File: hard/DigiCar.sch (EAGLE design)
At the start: 41 parts, among them CN1 EH-2, CN11 ZX62-B-5PA(11), CN2 EH-2, CN3 EH-2, Q1 2SC2712, Q2 2SC2712, SW1 SS-12SDP2, SW2 SKRPACE010, U1 TC1262-3.3VDB, U2 DRV8835, U3 ESP-WROOM-32, U4 FT231XS

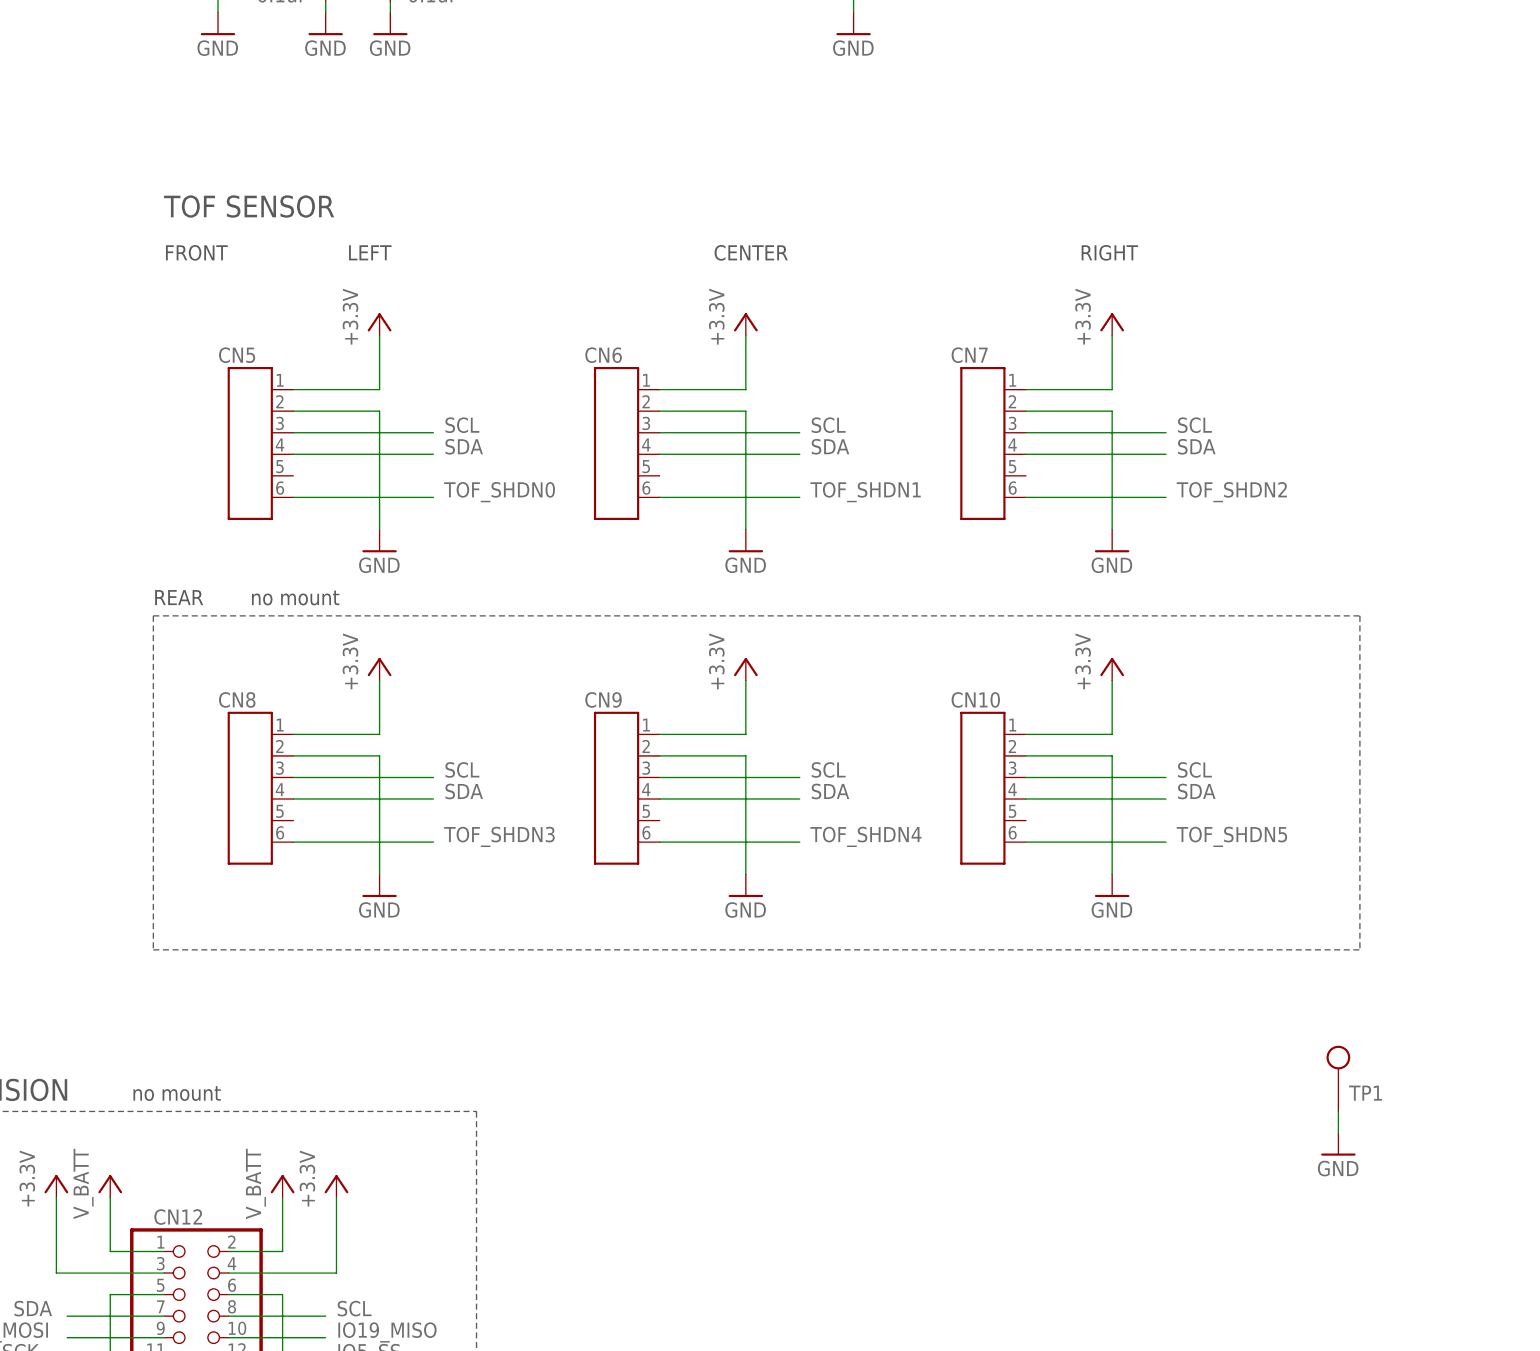
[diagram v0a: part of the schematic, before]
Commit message: 回路を修正
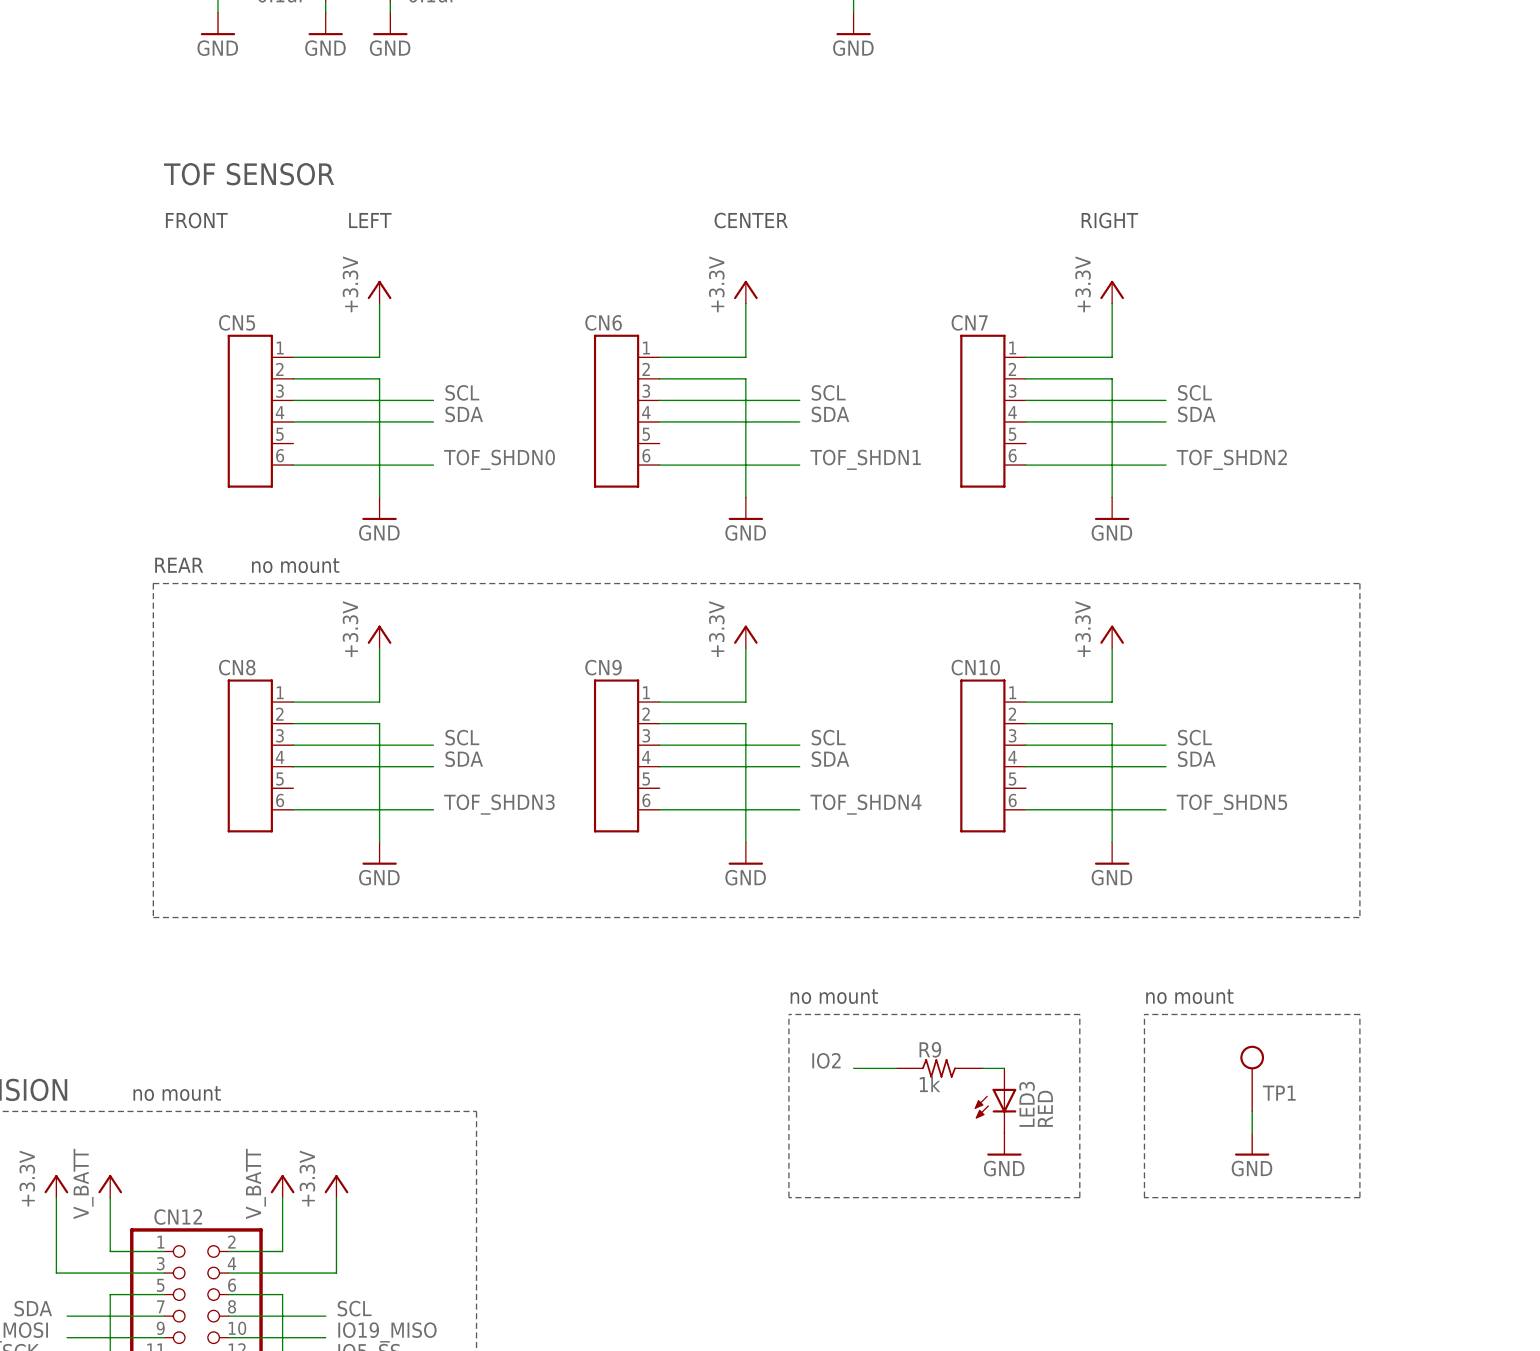
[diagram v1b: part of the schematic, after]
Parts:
- added LED3: RED, lipoyang_discrete:LED1608
- added R9: 1k, lipoyang_cr:R-CP-1608
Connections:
- new net N$2: LED3.A, R9.PIN2
- net GND: now also LED3.C
- net IO2: now also R9.PIN1
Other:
- moved on the sheet: CN10, CN5, CN6, CN7, CN8, CN9, TP1
